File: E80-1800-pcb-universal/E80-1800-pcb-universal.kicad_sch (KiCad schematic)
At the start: 48 parts, among them J1 SPI, J2 BATT, J3 OLED, J4 USB_C_Receptacle_USB2.0, Q1 Q_NMOS_GSD, SW1 RST, SW2 BOOT, U1 SRV05-4, U2 XC6206P332MR, U3 STM32F072RBTx

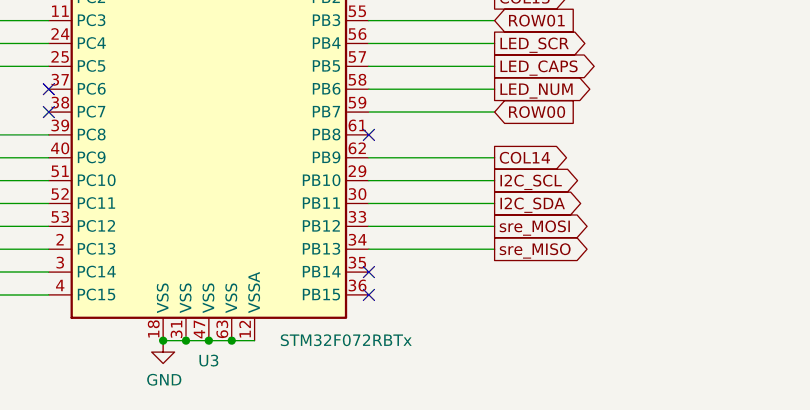
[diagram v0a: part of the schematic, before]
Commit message: prepare for jlcpcb
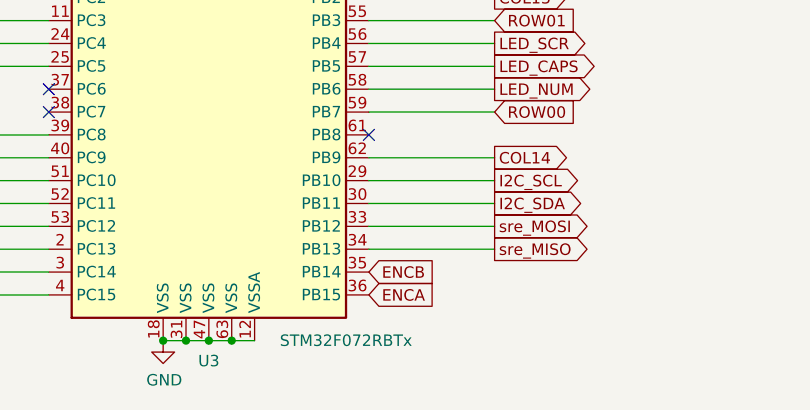
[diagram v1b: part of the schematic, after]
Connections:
- net ENCB: now reaches U3.35 (PB14)
- net ENCA: now reaches U3.36 (PB15)
- no-connect marks 9 -> 7
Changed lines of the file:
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@@
   (junction (at 25.4 138.43) (diameter 0) (color 0 0 0 0)
   )
-  (no_connect (at 106.68 186.69))
   (no_connect (at 106.68 130.81))
   (no_connect (at 106.68 140.97))
@@
   (no_connect (at 41.91 55.88))
   (no_connect (at 71.12 166.37))
-  (no_connect (at 106.68 184.15))
   (wire (pts (xy 233.68 60.96) (xy 243.84 60.96))
     (stroke (width 0) (type default) (color 0 0 0 0))
@@
     )
   )
+  (global_label "ENCA" (shape input) (at 106.68 186.69 0) (fields_autoplaced)
+    (effects (font (size 1.27 1.27)) (justify left))
+    (property "Intersheet References" "${INTERSHEET_REFS}" (id 0) (at 113.8423 186.6106 0)
+      (effects (font (size 1.27 1.27)) (justify left) hide)
+    )
+  )
   (global_label "SPI_IRQ" (shape input) (at 120.65 113.03 0) (fields_autoplaced)
     (effects (font (size 1.27 1.27)) (justify left))
@@
     )
   )
+  (global_label "ENCB" (shape input) (at 106.68 184.15 0) (fields_autoplaced)
+    (effects (font (size 1.27 1.27)) (justify left))
+    (property "Intersheet References" "${INTERSHEET_REFS}" (id 0) (at 114.0237 184.0706 0)
+      (effects (font (size 1.27 1.27)) (justify left) hide)
+    )
+  )
